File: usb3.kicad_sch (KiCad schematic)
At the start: 50 parts, among them J5 WE_632723300011_alt_symbol, Q19 PJE138K, Q4 PJE138K, U17 HD3SS3220, U18 AP22615, U19 TPD4E05U06QDQARQ1, U20 TPD4E05U06QDQARQ1, U21 TPD4E05U06QDQARQ1

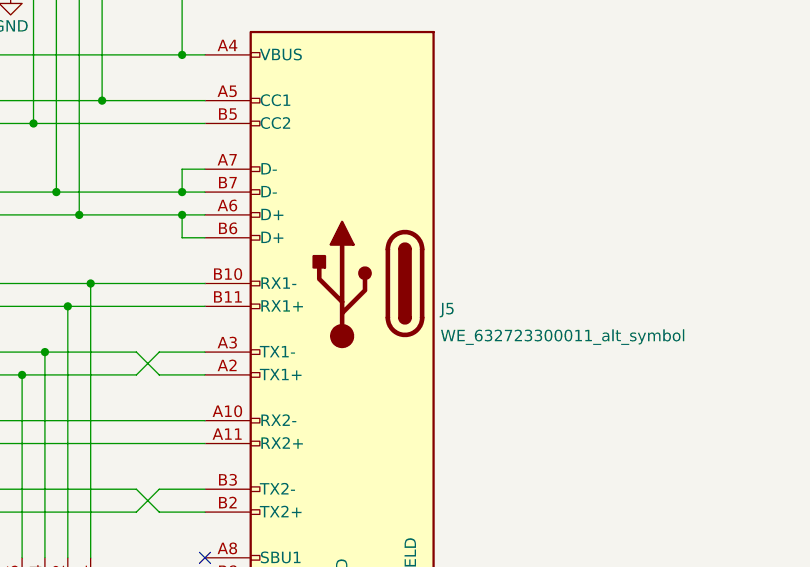
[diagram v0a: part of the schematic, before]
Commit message: Simplification continues
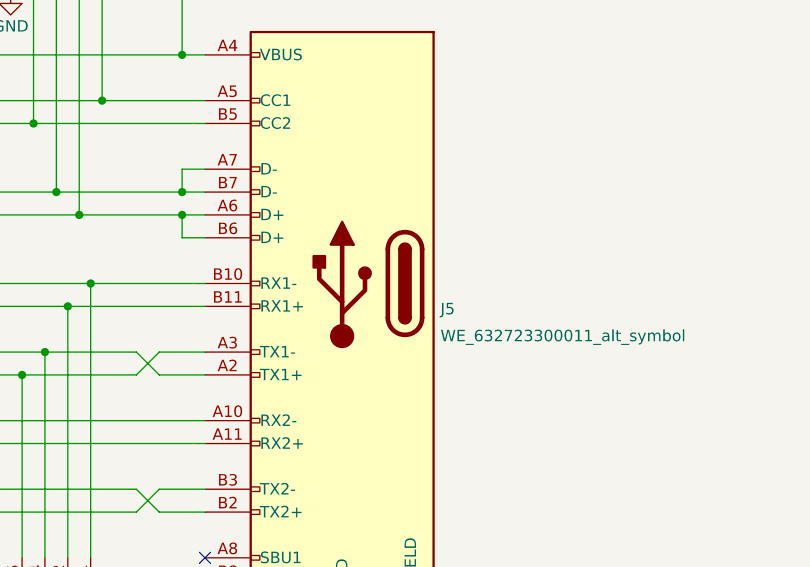
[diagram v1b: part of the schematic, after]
